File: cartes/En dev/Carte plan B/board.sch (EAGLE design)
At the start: 21 parts

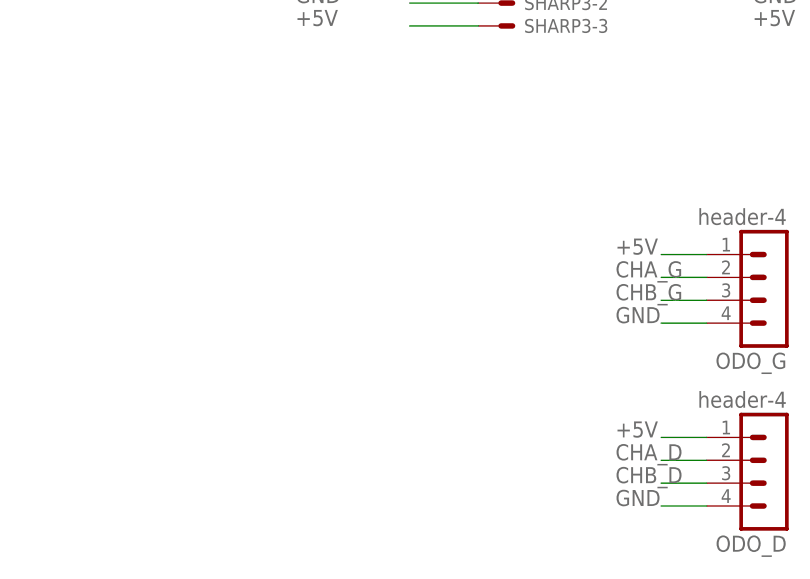
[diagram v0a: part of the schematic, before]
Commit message: nouveaux gerber
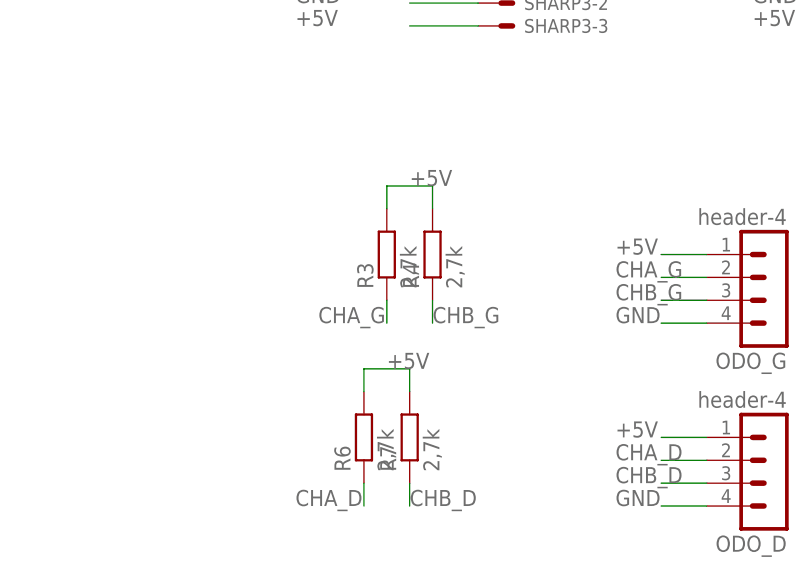
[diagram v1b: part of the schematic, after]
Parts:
- added R3, R4, R6, R7: 2,7k, rcl:R-EU_R0805
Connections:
- net +5V: now also R3.2, R4.2, R6.2, R7.2
- net CHA_D: now also R6.1
- net CHA_G: now also R3.1
- net CHB_D: now also R7.1
- net CHB_G: now also R4.1
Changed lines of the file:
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@@
 <part name="+5V" library="supply1" deviceset="VCC" device="" value="+5v"/>
 <part name="GND2" library="supply1" deviceset="GND" device=""/>
+<part name="R3" library="rcl" deviceset="R-EU_" device="R0805" value="2,7k"/>
+<part name="R4" library="rcl" deviceset="R-EU_" device="R0805" value="2,7k"/>
+<part name="R6" library="rcl" deviceset="R-EU_" device="R0805" value="2,7k"/>
+<part name="R7" library="rcl" deviceset="R-EU_" device="R0805" value="2,7k"/>
 </parts>
 <sheets>
@@
 <instance part="+5V" gate="VCC" x="318.77" y="77.47" rot="R180"/>
 <instance part="GND2" gate="1" x="340.36" y="77.47"/>
+<instance part="R3" gate="G$1" x="147.32" y="43.18" rot="R90"/>
+<instance part="R4" gate="G$1" x="152.4" y="43.18" rot="R90"/>
+<instance part="R6" gate="G$1" x="144.78" y="22.86" rot="R90"/>
+<instance part="R7" gate="G$1" x="149.86" y="22.86" rot="R90"/>
 </instances>
 <busses>
@@
 <pinref part="+5V" gate="VCC" pin="VCC"/>
 </segment>
+<segment>
+<pinref part="R3" gate="G$1" pin="2"/>
+<wire x1="147.32" y1="48.26" x2="147.32" y2="50.8" width="0.1524" layer="91"/>
+<pinref part="R4" gate="G$1" pin="2"/>
+<wire x1="152.4" y1="48.26" x2="152.4" y2="50.8" width="0.1524" layer="91"/>
+<wire x1="147.32" y1="50.8" x2="152.4" y2="50.8" width="0.1524" layer="91"/>
+<label x="149.86" y="50.8" size="1.778" layer="95"/>
+</segment>
+<segment>
+<pinref part="R6" gate="G$1" pin="2"/>
+<wire x1="144.78" y1="27.94" x2="144.78" y2="30.48" width="0.1524" layer="91"/>
+<pinref part="R7" gate="G$1" pin="2"/>
+<wire x1="149.86" y1="27.94" x2="149.86" y2="30.48" width="0.1524" layer="91"/>
+<wire x1="144.78" y1="30.48" x2="149.86" y2="30.48" width="0.1524" layer="91"/>
+<label x="147.32" y="30.48" size="1.778" layer="95"/>
+</segment>
 </net>
 <net name="CANL" class="0">
@@
 <label x="279.4" y="139.7" size="1.778" layer="95"/>
 </segment>
+<segment>
+<pinref part="R3" gate="G$1" pin="1"/>
+<wire x1="147.32" y1="38.1" x2="147.32" y2="35.56" width="0.1524" layer="91"/>
+<label x="139.7" y="35.56" size="1.778" layer="95"/>
+</segment>
 </net>
 <net name="CHB_G" class="0">
@@
 <label x="279.4" y="142.24" size="1.778" layer="95"/>
 </segment>
+<segment>
+<pinref part="R4" gate="G$1" pin="1"/>
+<wire x1="152.4" y1="38.1" x2="152.4" y2="35.56" width="0.1524" layer="91"/>
+<label x="152.4" y="35.56" size="1.778" layer="95"/>
+</segment>
 </net>
 <net name="CHA_D" class="0">
@@
 <label x="165.1" y="142.24" size="1.778" layer="95"/>
 </segment>
+<segment>
+<pinref part="R6" gate="G$1" pin="1"/>
+<wire x1="144.78" y1="17.78" x2="144.78" y2="15.24" width="0.1524" layer="91"/>
+<label x="137.16" y="15.24" size="1.778" layer="95"/>
+</segment>
 </net>
 <net name="CHB_D" class="0">
@@
 <label x="165.1" y="139.7" size="1.778" layer="95"/>
 </segment>
-</net>
+<segment>
+<pinref part="R7" gate="G$1" pin="1"/>
+<wire x1="149.86" y1="17.78" x2="149.86" y2="15.24" width="0.1524" layer="91"/>
+<label x="149.86" y="15.24" size="1.778" layer="95"/>
+</segment>
+</net>
